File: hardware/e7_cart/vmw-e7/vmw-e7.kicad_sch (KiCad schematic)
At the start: 6 parts, among them U1 2600Cartridge, U2 ROM, U3 ROM, U4 SRAM, U5 E7

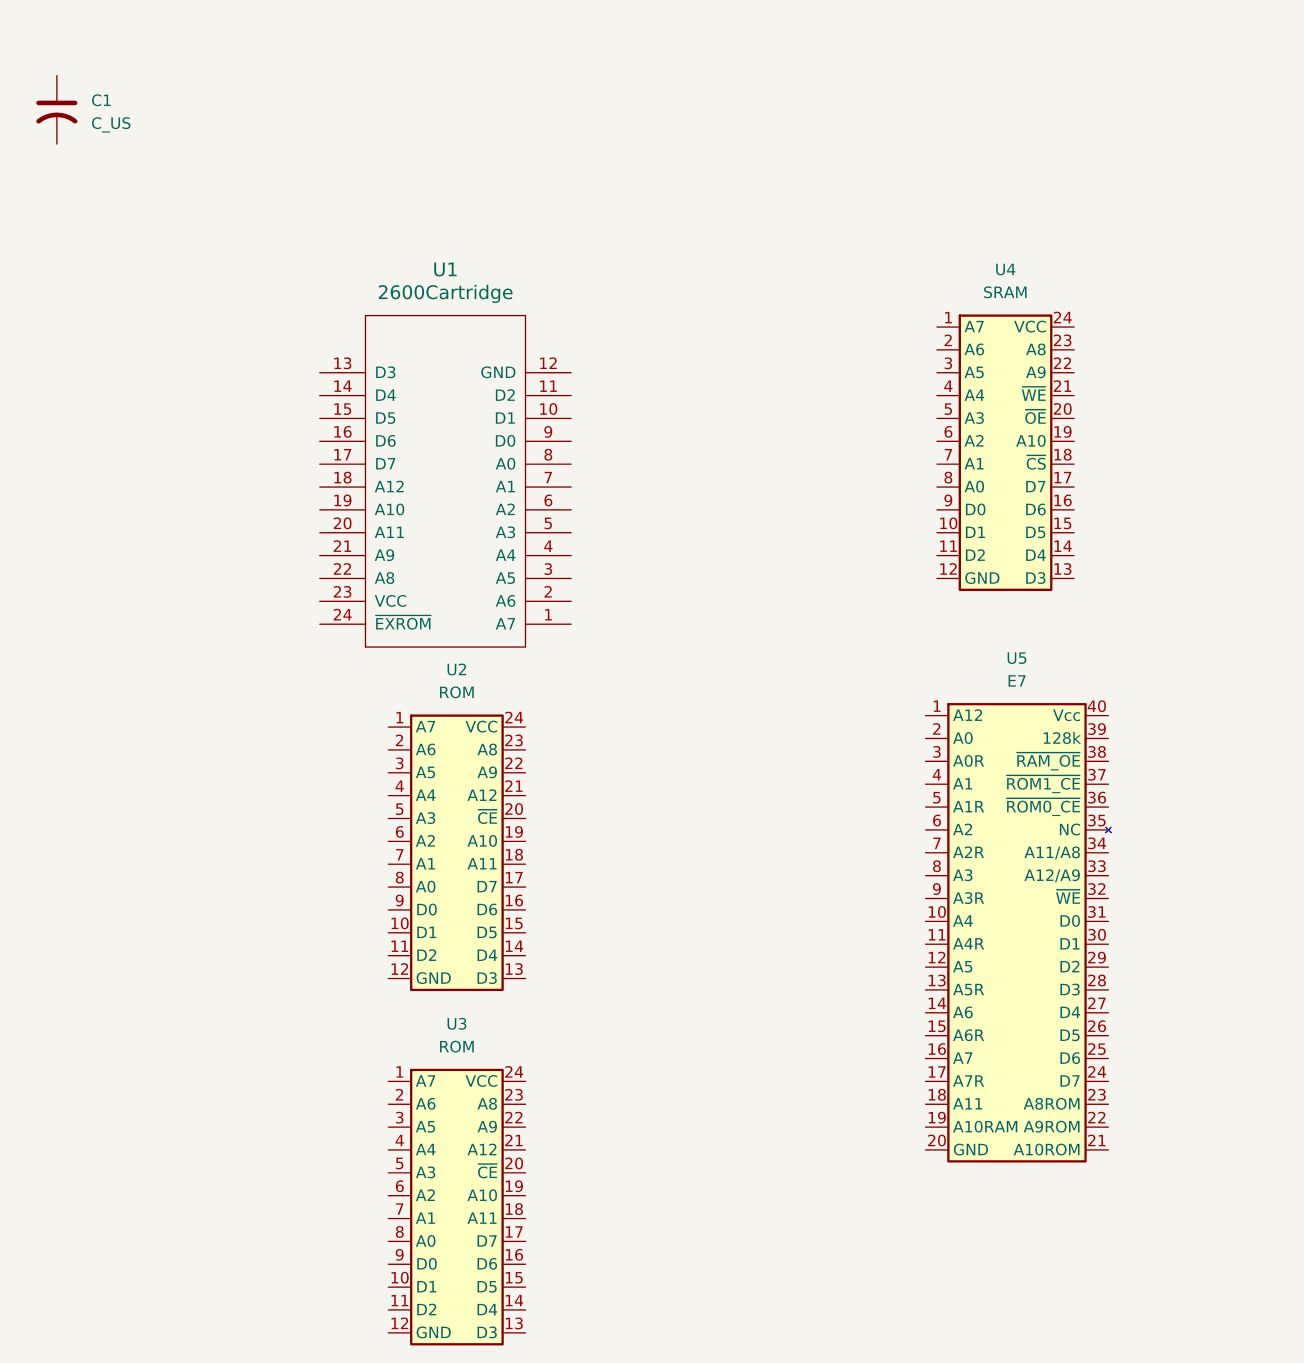
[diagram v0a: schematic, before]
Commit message: e7: more work on schematic
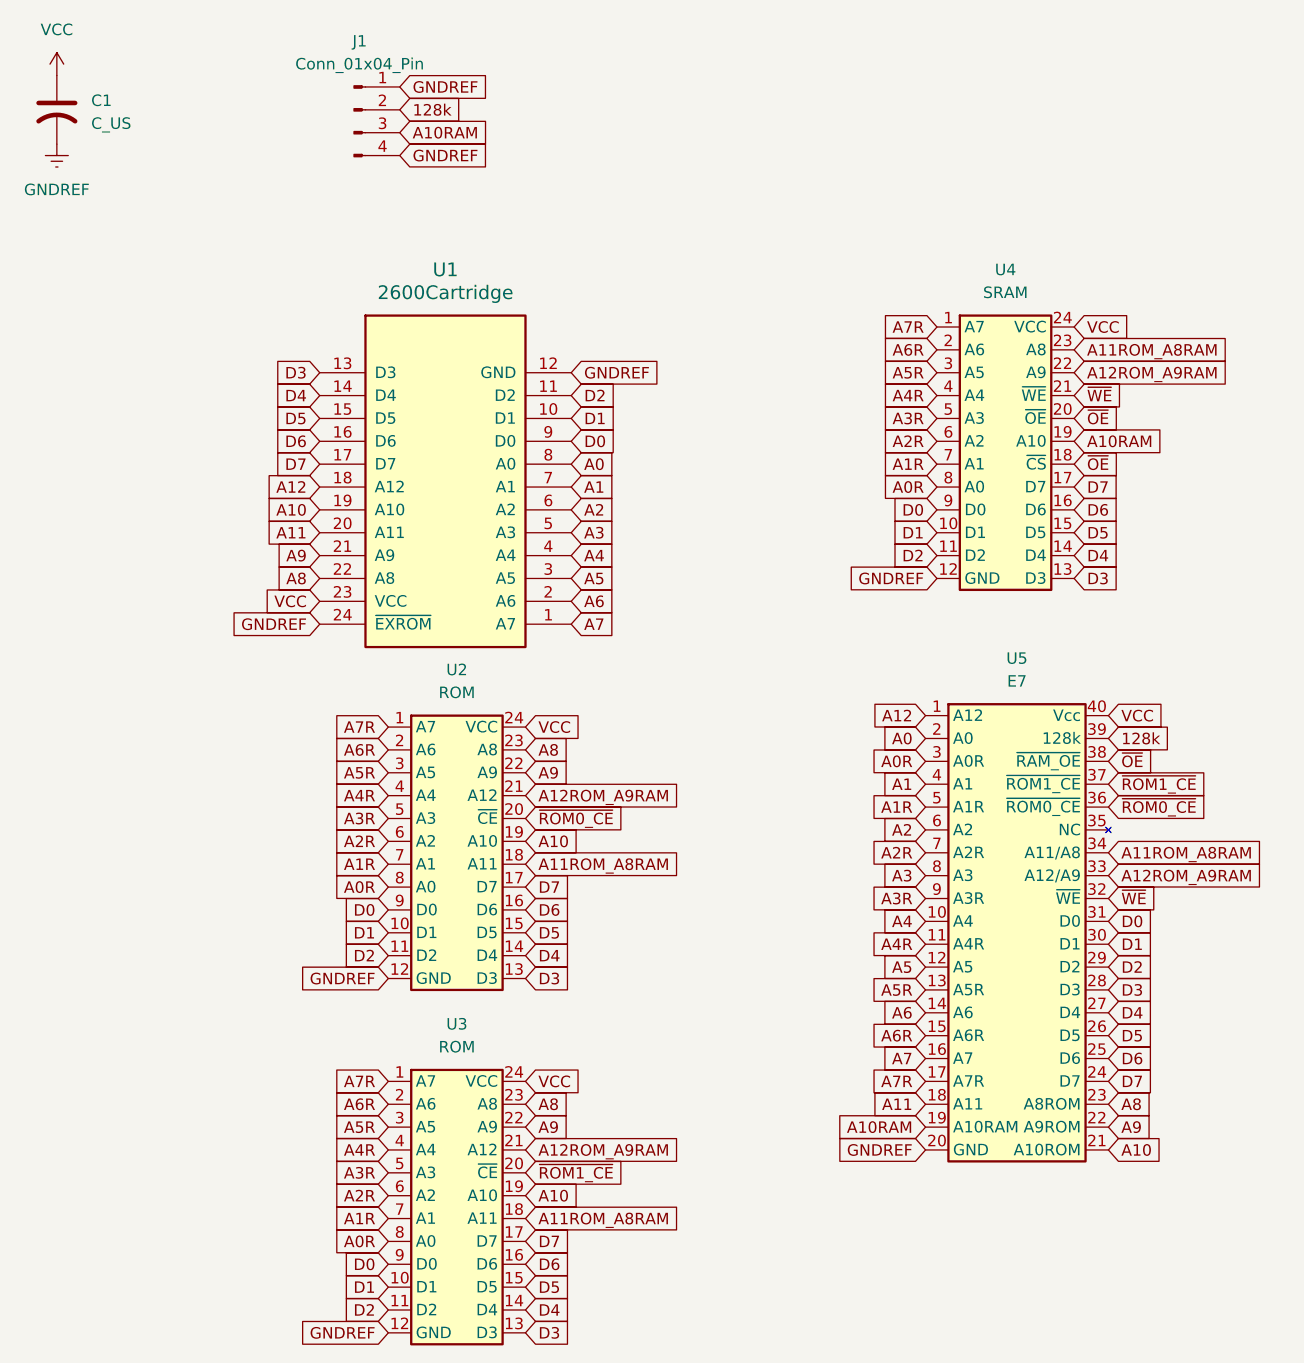
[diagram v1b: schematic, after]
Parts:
- added J1: Conn_01x04_Pin, symbol Connector:Conn_01x04_Pin
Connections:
- net A7: now reaches U1.1 (A7)
- net A7: now also U5.16 (A7)
- net D1: now reaches U1.10 (D1)
- net D1: now also U2.10 (D1), U3.10 (D1), U4.10 (D1), U5.30 (D1)
- net D2: now reaches U1.11 (D2)
- net D2: now also U2.11 (D2), U3.11 (D2), U4.11 (D2), U5.29 (D2)
- net GNDREF: now reaches U1.12 (GND)
- net GNDREF: now also C1.2, U1.24 (~{EXROM}), U2.12 (GND), U3.12 (GND), U4.12 (GND), U5.20 (GND), J1.1 (Pin_1), J1.4 (Pin_4)
- net D3: now reaches U1.13 (D3)
- net D3: now also U2.13 (D3), U3.13 (D3), U4.13 (D3), U5.28 (D3)
- net D4: now reaches U1.14 (D4)
- net D4: now also U2.14 (D4), U3.14 (D4), U4.14 (D4), U5.27 (D4)
- net D5: now reaches U1.15 (D5)
- net D5: now also U2.15 (D5), U3.15 (D5), U4.15 (D5), U5.26 (D5)
- net D6: now reaches U1.16 (D6)
- net D6: now also U2.16 (D6), U3.16 (D6), U4.16 (D6), U5.25 (D6)
- net D7: now reaches U1.17 (D7)
- net D7: now also U2.17 (D7), U3.17 (D7), U4.17 (D7), U5.24 (D7)
- net A12: now reaches U1.18 (A12)
- net A12: now also U5.1 (A12)
- net A10: now reaches U1.19 (A10)
- net A10: now also U2.19 (A10), U3.19 (A10), U5.21 (A10ROM)
- net A6: now reaches U1.2 (A6)
- net A6: now also U5.14 (A6)
- net A11: now reaches U1.20 (A11)
- net A11: now also U5.18 (A11)
- net A9: now reaches U1.21 (A9)
- net A9: now also U2.22 (A9), U3.22 (A9), U5.22 (A9ROM)
- net A8: now reaches U1.22 (A8)
- net A8: now also U2.23 (A8), U3.23 (A8), U5.23 (A8ROM)
- net VCC: now reaches U1.23 (VCC)
- net VCC: now also C1.1, U2.24 (VCC), U3.24 (VCC), U4.24 (VCC), U5.40 (Vcc)
- net A5: now reaches U1.3 (A5)
- net A5: now also U5.12 (A5)
- net A4: now reaches U1.4 (A4)
- net A4: now also U5.10 (A4)
- net A3: now reaches U1.5 (A3)
- net A3: now also U5.8 (A3)
- net A2: now reaches U1.6 (A2)
- net A2: now also U5.6 (A2)
- net A1: now reaches U1.7 (A1)
- net A1: now also U5.4 (A1)
- net A0: now reaches U1.8 (A0)
- net A0: now also U5.2 (A0)
- net D0: now reaches U1.9 (D0)
- net D0: now also U2.9 (D0), U3.9 (D0), U4.9 (D0), U5.31 (D0)
- net A7R: now reaches U2.1 (A7)
- net A7R: now also U3.1 (A7), U4.1 (A7), U5.17 (A7R)
- net A11ROM_A8RAM: now reaches U2.18 (A11)
- net A11ROM_A8RAM: now also U3.18 (A11), U4.23 (A8), U5.34 (A11/A8)
- net A6R: now reaches U2.2 (A6)
- net A6R: now also U3.2 (A6), U4.2 (A6), U5.15 (A6R)
- net ~{ROM0_CE}: now reaches U2.20 (~{CE})
- net ~{ROM0_CE}: now also U5.36 (~{ROM0_CE})
- net A12ROM_A9RAM: now reaches U2.21 (A12)
- net A12ROM_A9RAM: now also U3.21 (A12), U4.22 (A9), U5.33 (A12/A9)
- net A5R: now reaches U2.3 (A5)
- net A5R: now also U3.3 (A5), U4.3 (A5), U5.13 (A5R)
- net A4R: now reaches U2.4 (A4)
- net A4R: now also U3.4 (A4), U4.4 (A4), U5.11 (A4R)
- net A3R: now reaches U2.5 (A3)
- net A3R: now also U3.5 (A3), U4.5 (A3), U5.9 (A3R)
- net A2R: now reaches U2.6 (A2)
- net A2R: now also U3.6 (A2), U4.6 (A2), U5.7 (A2R)
- net A1R: now reaches U2.7 (A1)
- net A1R: now also U3.7 (A1), U4.7 (A1), U5.5 (A1R)
- net A0R: now reaches U2.8 (A0)
- net A0R: now also U3.8 (A0), U4.8 (A0), U5.3 (A0R)
- net A10RAM: now reaches U5.19 (A10RAM)
- net A10RAM: now also U4.19 (A10), J1.3 (Pin_3)
- net ~{WE}: now reaches U5.32 (~{WE})
- net ~{WE}: now also U4.21 (~{WE})
- net ~{ROM1_CE}: now reaches U5.37 (~{ROM1_CE})
- net ~{ROM1_CE}: now also U3.20 (~{CE})
- net ~{OE}: now reaches U5.38 (~{RAM_OE})
- net ~{OE}: now also U4.18 (~{CS}), U4.20 (~{OE})
- net 128k: now reaches U5.39 (128k)
- net 128k: now also J1.2 (Pin_2)
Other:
- company: (none) -> VMW Hardware Productions
- title: (none) -> VMW E7 Cartridge

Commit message: e7: update hardware
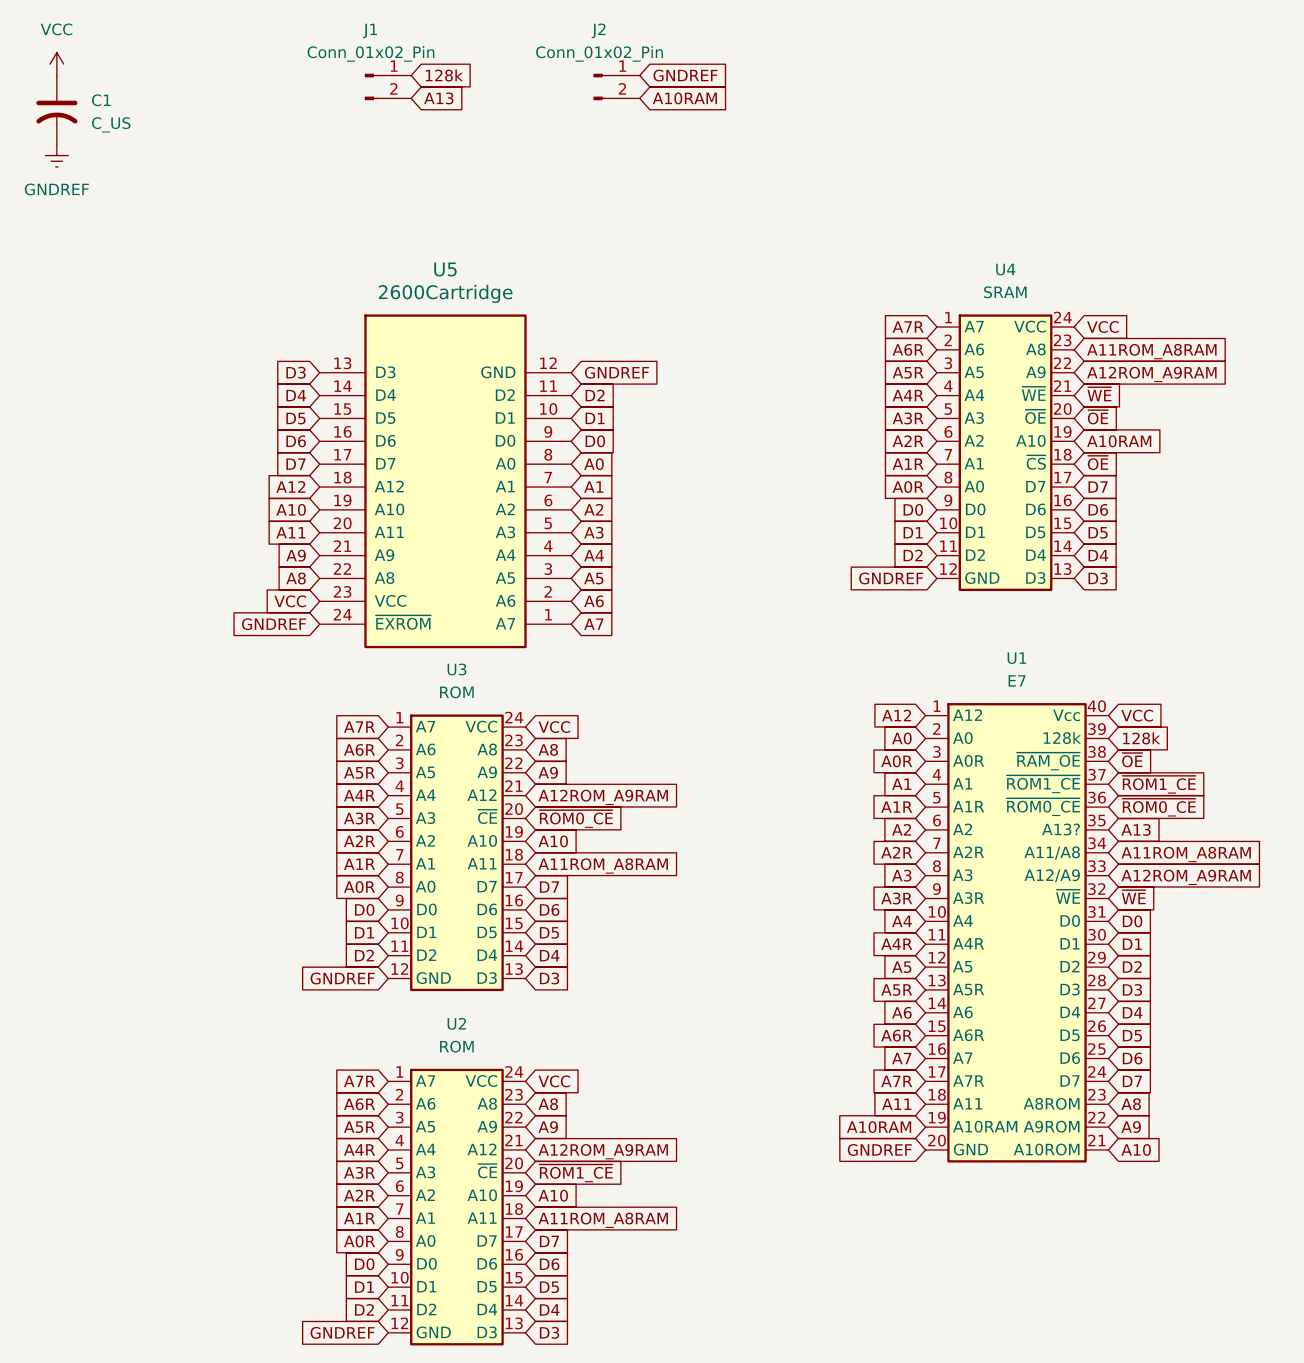
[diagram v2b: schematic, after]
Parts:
- removed J1: Conn_01x04_Pin, symbol Connector:Conn_01x04_Pin
- added J1, J2: Conn_01x02_Pin, Connector_PinHeader_2.54mm:PinHeader_1x02_P2.54mm_Vertical, symbol Connector:Conn_01x02_Pin
- C1: footprint (none) -> Capacitor_THT:C_Disc_D3.0mm_W1.6mm_P2.50mm
- U1: renamed from U5; footprint (none) -> Package_DIP:DIP-40_W15.24mm_Socket
- U2: renamed from U3; footprint (none) -> Package_DIP:DIP-24_W15.24mm
- U3: renamed from U2; footprint (none) -> Package_DIP:DIP-24_W15.24mm
- U4: footprint (none) -> Package_DIP:DIP-24_W15.24mm
- U5: renamed from U1; footprint (none) -> atari2600:2600CART
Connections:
- net 128k: now also J1.1 (Pin_1)
- net A10RAM: now also J2.2 (Pin_2)
- net GNDREF: now also J2.1 (Pin_1)
- net A13: now reaches U1.35 (A13?)
- net A13: now also J1.2 (Pin_2)
